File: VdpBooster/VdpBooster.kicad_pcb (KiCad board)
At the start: 2 copper layers, 36.2 x 73 mm, 30 parts, among them U1 M5M4C264L, U2 M5M4C264L, U3 M5M4C264L, U4 M5M4C264L, U5 315-5313A

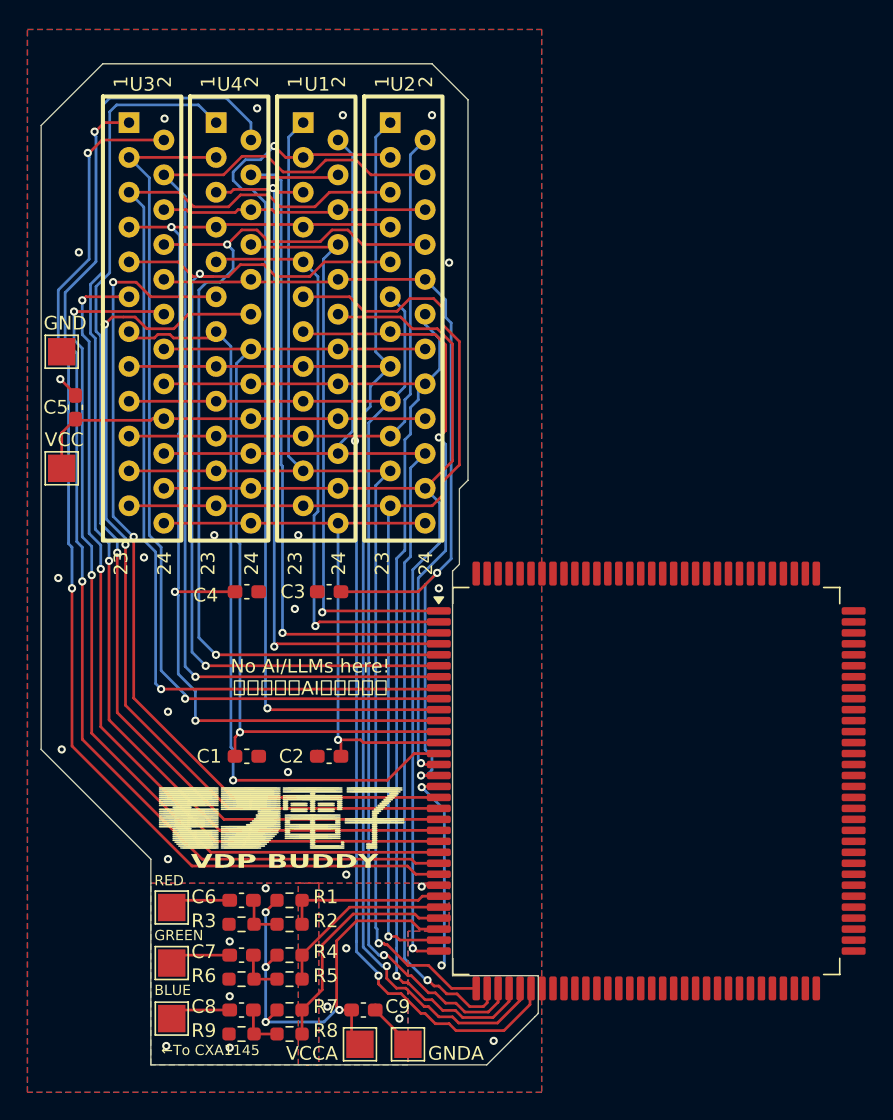
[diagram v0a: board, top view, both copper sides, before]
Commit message: v101 changes
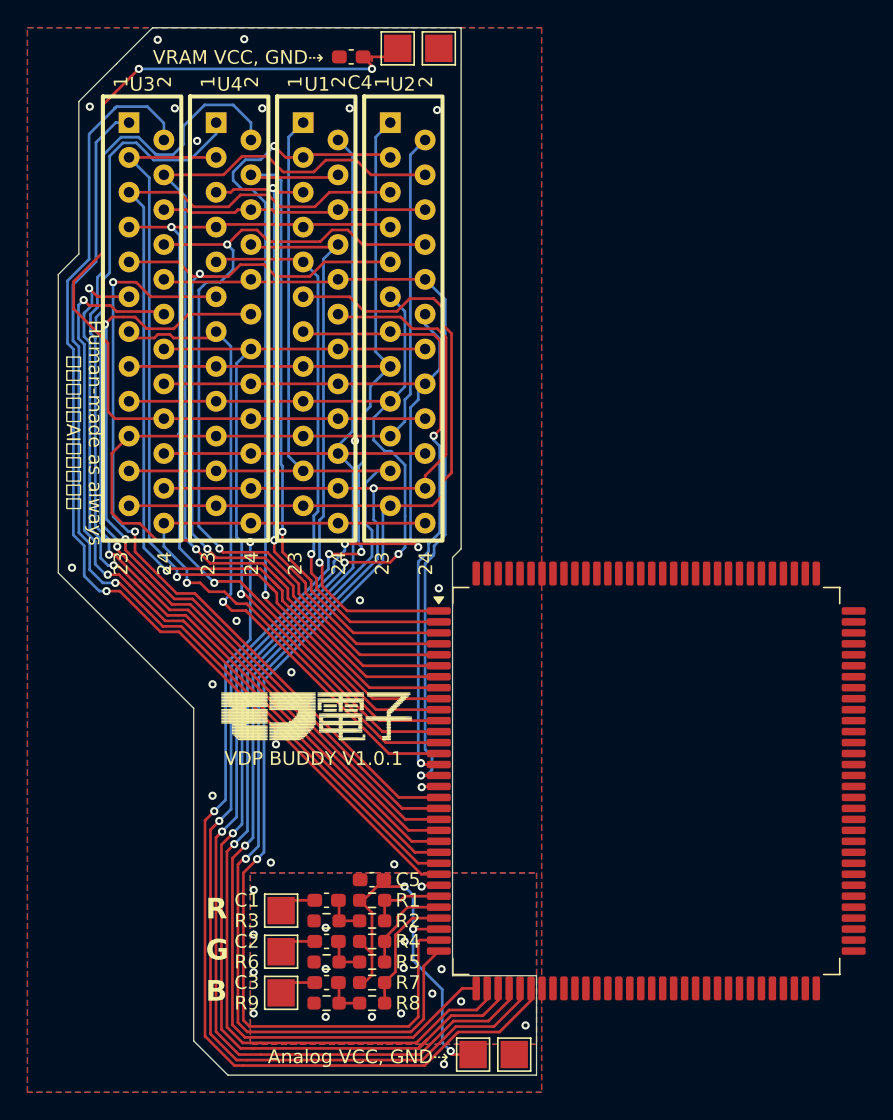
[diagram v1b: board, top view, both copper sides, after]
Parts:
- removed the C1 at (131.0, 65.5)
- removed the C2 at (137.0, 65.5)
- removed the C3 at (137.0, 53.5)
- removed the C4 at (131.0, 53.5)
- moved TP3 39.2 mm to (142.0, 13.9)
- moved TP4 35.3 mm to (145.0, 13.9)
- moved C4 32.5 mm to (138.6, 14.5), turned to 180 degrees
- moved C5 9.52 mm to (140.1, 74.5), turned to 180 degrees
- moved TP1 8.28 mm to (147.5, 87.2)
- moved TP7 8.19 mm to (133.5, 82.8)
- moved TP6 8.02 mm to (133.5, 79.8)
- moved TP5 7.98 mm to (133.5, 76.8)
- moved TP2 7.79 mm to (150.5, 87.2)
- moved R9 6.60 mm to (136.8, 83.5)
- moved C3 6.51 mm to (136.8, 82.0)
- moved R8 6.43 mm to (140.1, 83.5)
- moved R7 6.35 mm to (140.1, 82.0)
- moved R6 6.32 mm to (136.8, 80.5)
- moved C2 6.28 mm to (136.8, 79.0)
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- renumbered C6 to C1, C7 to C2, C8 to C3, C5 to C4, C9 to C5
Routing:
- net VCC: track 29.6 -> 72.8 mm, vias 0 -> 2
- net /A7: track 96.4 -> 123.9 mm, vias 2 -> 3
- net /A5: track 80.0 -> 107.1 mm, vias 1 -> 3
- net /A0: track 84.4 -> 110.9 mm
- net /A4: track 80.6 -> 106.5 mm, vias 1 -> 3
- net /A1: track 76.4 -> 102.3 mm, vias 1 -> 2
- net /A2: track 88.8 -> 111.7 mm
- net /A6: track 96.7 -> 119.3 mm, vias 1 -> 3
- net /A3: track 88.9 -> 110.5 mm
- net GND: track 36.5 -> 20.7 mm, vias 21 -> 20
- net /SC: track 78.5 -> 67.3 mm, vias 3 -> 2
- net /RD6: track 78.3 -> 69.7 mm, vias 2 -> 1
- net /RD2: track 80.0 -> 71.6 mm
- net /~{WE1}: track 56.0 -> 47.7 mm
- net /~{OE1}: track 66.8 -> 58.8 mm, vias 2 -> 1
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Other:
- board size 36.2 x 73 mm -> 34.9 x 76.4 mm
- board text added: "Analog VCC, GND⇢"
- board text added: "B"
- board text added: "G"
- board text added: "Human-made as always いつも通りAI不使用です"
- board text added: "R"
- board text added: "VDP BUDDY V1.0.1"
- board text added: "VRAM VCC, GND⇢"
- board text removed: "BLUE"
- board text removed: "GND"
- board text removed: "GNDA"
- board text removed: "GREEN"
- board text removed: "No AI/LLMs here! いつも通りAI不使用です"
- board text removed: "RED"
- board text removed: "VCC"
- board text removed: "VCCA"
- board text removed: "VDP BUDDY"
- board text removed: "←To CXA1145"

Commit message: tweaks and gerbils
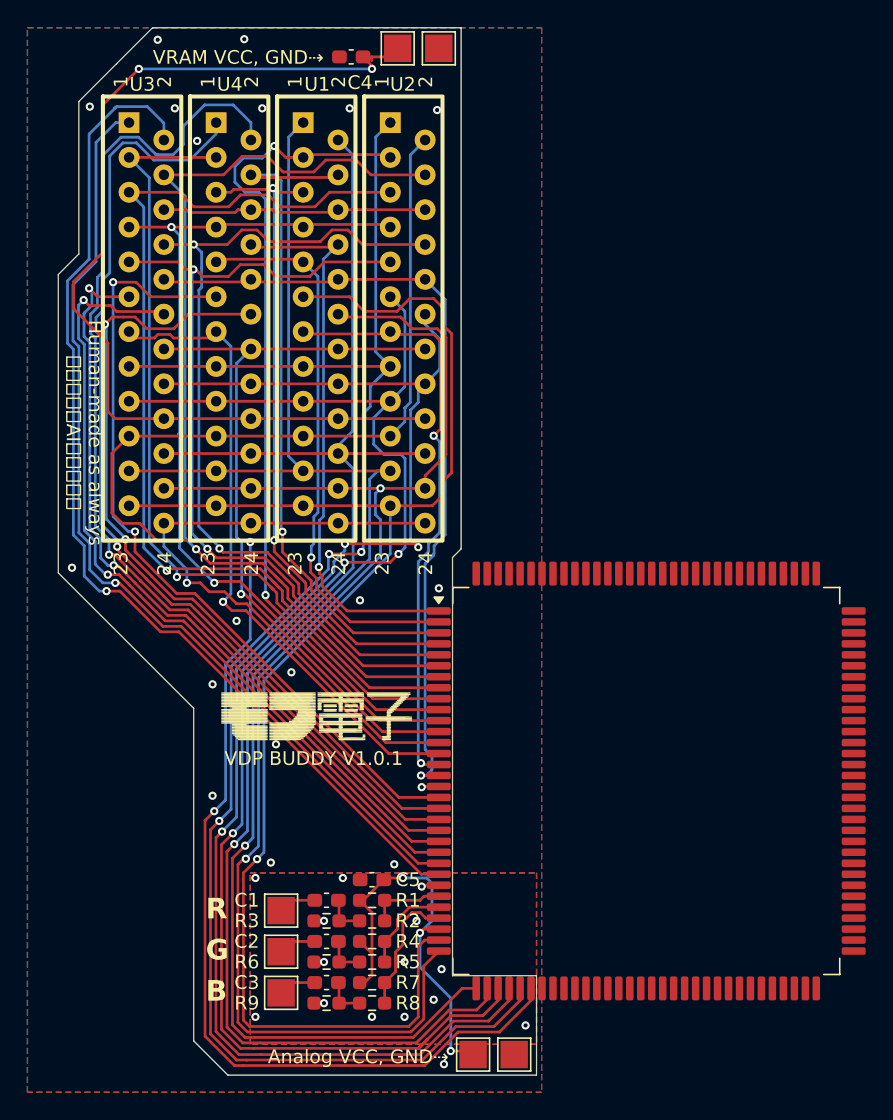
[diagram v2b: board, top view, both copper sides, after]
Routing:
- net /SD4: track 65.2 -> 63.7 mm
- net /SD5: track 63.4 -> 62.5 mm
- net VCCA: track 30.2 -> 31.1 mm
- net /VID_B: track 8.97 -> 9.55 mm
- net /A7: track 123.9 -> 123.7 mm, vias 3 -> 2
- net GNDA: vias 16 -> 14
